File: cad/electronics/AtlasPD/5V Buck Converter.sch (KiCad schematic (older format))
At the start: 16 parts, among them U1 LM2678T-ADJ_NOPB, U5 AMS1117-3.3

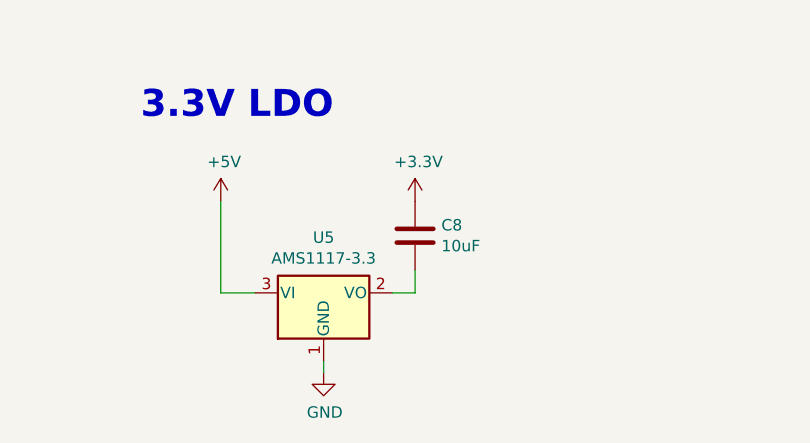
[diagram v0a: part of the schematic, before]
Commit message: Found a bug, squashed it
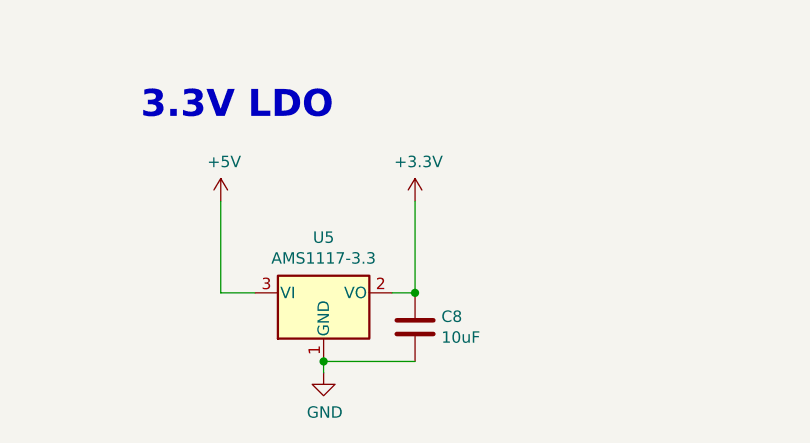
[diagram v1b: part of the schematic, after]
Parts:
- C8: footprint Capacitor_SMD:C_0805_2012Metric -> Capacitor_SMD:C_0603_1608Metric
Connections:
- wire segments 55 -> 56
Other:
- moved on the sheet: C8
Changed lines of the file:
@@
 	2450 4200 2550 4200
-Wire Wire Line
-	2550 4200 2550 4100
 Wire Wire Line
 	2150 4500 2150 4550
@@
 L Device:C C8
 U 1 1 6163B27F
-P 2550 3950
-F 0 "C8" H 2665 3996 50  0000 L CNN
-F 1 "10uF" H 2665 3905 50  0000 L CNN
-F 2 "Capacitor_SMD:C_0805_2012Metric" H 2588 3800 50  0001 C CNN
-F 3 "~" H 2550 3950 50  0001 C CNN
-	1    2550 3950
+P 2550 4350
+F 0 "C8" H 2665 4396 50  0000 L CNN
+F 1 "10uF" H 2665 4305 50  0000 L CNN
+F 2 "Capacitor_SMD:C_0603_1608Metric" H 2588 4200 50  0001 C CNN
+F 3 "~" H 2550 4350 50  0001 C CNN
+	1    2550 4350
 	1    0    0    -1
 $EndComp
@@
 Connection ~ 1650 2650
 $Comp
-L power:+BATT #PWR?
+L power:+BATT #PWR0109
 U 1 1 616386ED
 P 1050 1550
-F 0 "#PWR?" H 1050 1400 50  0001 C CNN
+F 0 "#PWR0109" H 1050 1400 50  0001 C CNN
 F 1 "+BATT" H 1065 1723 50  0000 C CNN
 F 2 "" H 1050 1550 50  0001 C CNN
@@
 	1050 1550 1050 1700
 Connection ~ 1050 1700
+Connection ~ 2550 4200
+Wire Wire Line
+	2550 3800 2550 4200
+Wire Wire Line
+	2550 4500 2150 4500
+Connection ~ 2150 4500
 $EndSCHEMATC
